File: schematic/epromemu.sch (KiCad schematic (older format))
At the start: 10 parts, among them J1 EPROM Connector, U1 Teensy4.1, U2 74HC245, U3 74HC245, U4 74HC245, U5 74HC245

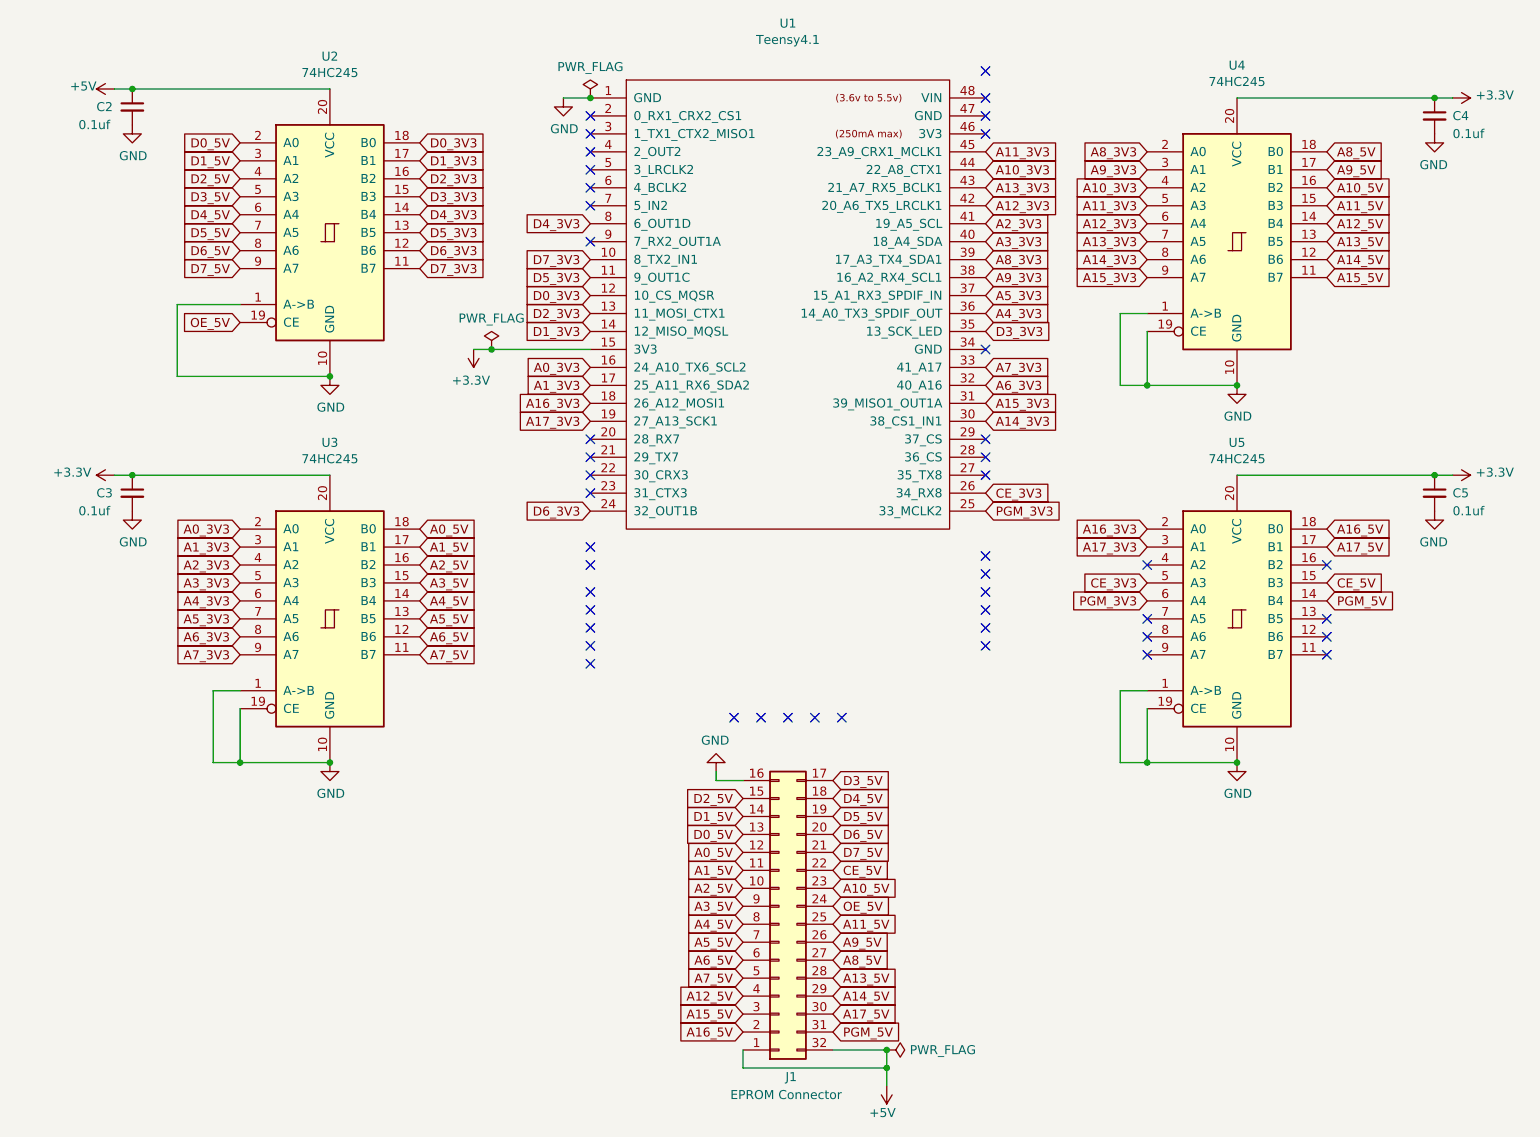
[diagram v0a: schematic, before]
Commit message: updates'
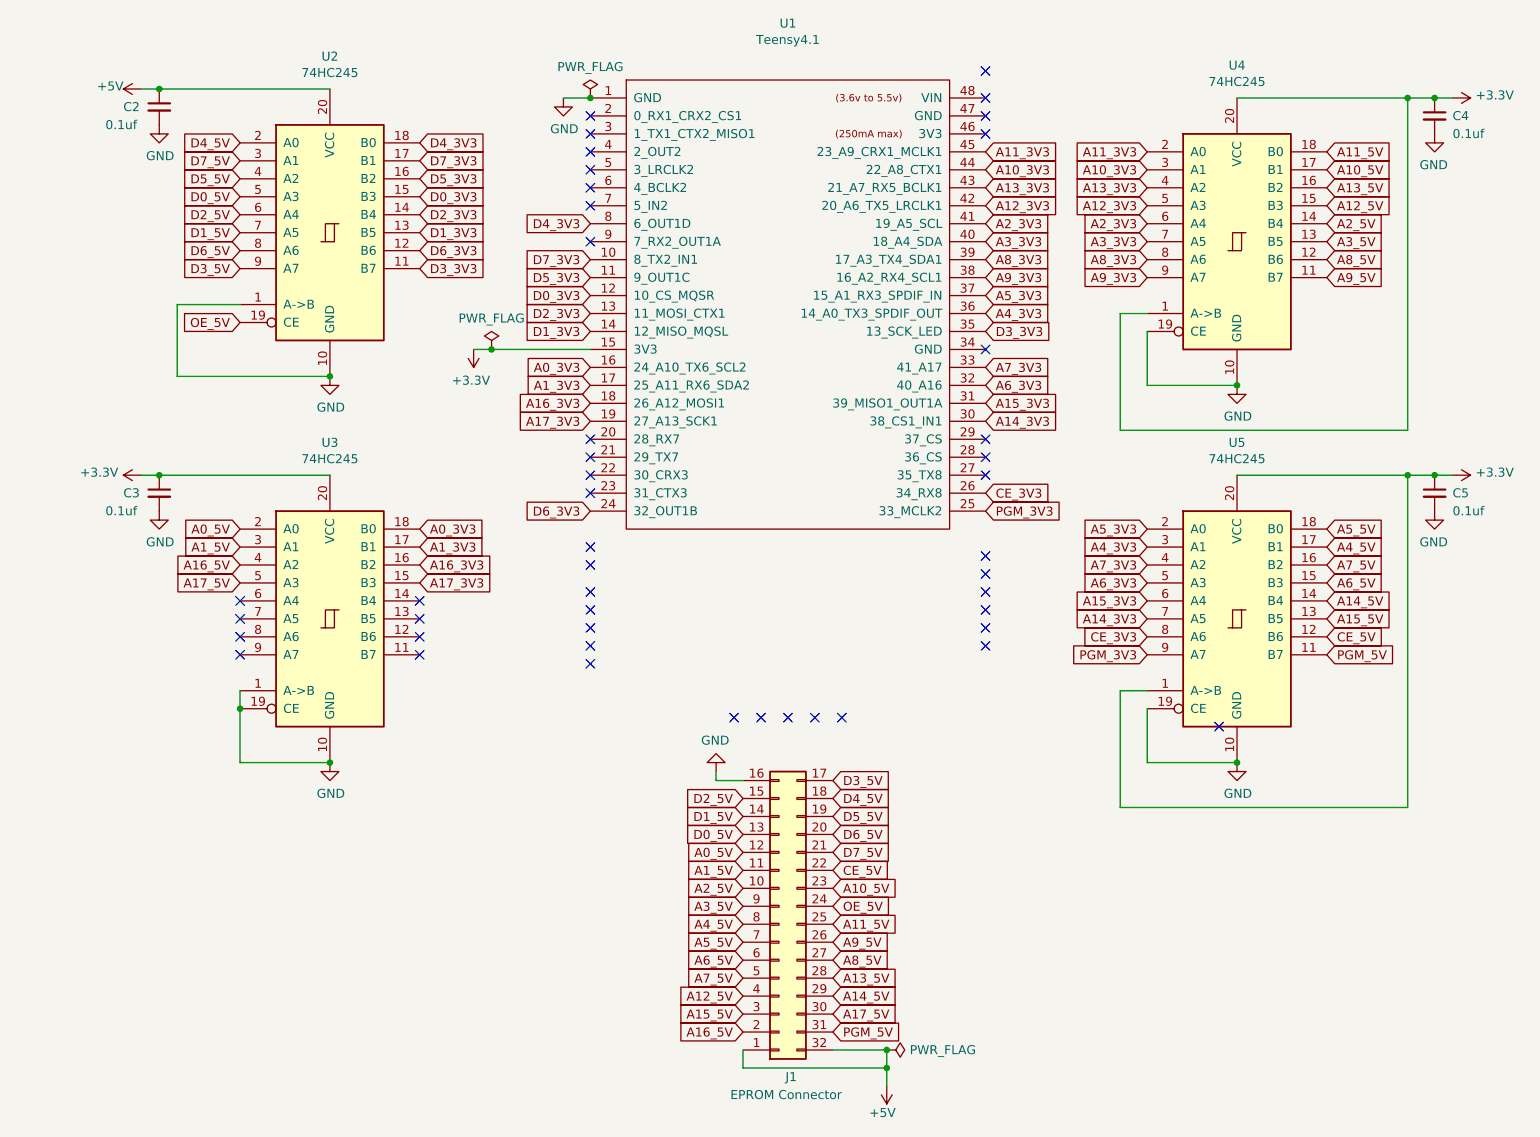
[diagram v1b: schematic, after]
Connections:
- net +3V3: now also U4.1 (A->B), U5.1 (A->B)
- net A0_3V3: now also U3.18 (B0); no longer U3.2 (A0)
- net A0_5V: now also U3.2 (A0); no longer U3.18 (B0)
- net A10_3V3: now also U4.3 (A1); no longer U4.4 (A2)
- net A10_5V: now also U4.17 (B1); no longer U4.16 (B2)
- net A11_3V3: now also U4.2 (A0); no longer U4.5 (A3)
- net A11_5V: now also U4.18 (B0); no longer U4.15 (B3)
- net A12_3V3: now also U4.5 (A3); no longer U4.6 (A4)
- net A12_5V: now also U4.15 (B3); no longer U4.14 (B4)
- net A13_3V3: now also U4.4 (A2); no longer U4.7 (A5)
- net A13_5V: now also U4.16 (B2); no longer U4.13 (B5)
- net A14_3V3: now also U5.7 (A5); no longer U4.8 (A6)
- net A14_5V: now also U5.14 (B4); no longer U4.12 (B6)
- net A15_3V3: now also U5.6 (A4); no longer U4.9 (A7)
- net A15_5V: now also U5.13 (B5); no longer U4.11 (B7)
- net A16_3V3: now also U3.16 (B2); no longer U5.2 (A0)
- net A16_5V: now also U3.4 (A2); no longer U5.18 (B0)
- net A17_3V3: now also U3.15 (B3); no longer U5.3 (A1)
- net A17_5V: now also U3.5 (A3); no longer U5.17 (B1)
- net A1_3V3: now also U3.17 (B1); no longer U3.3 (A1)
- net A1_5V: now also U3.3 (A1); no longer U3.17 (B1)
- net A2_3V3: now also U4.6 (A4); no longer U3.4 (A2)
- net A2_5V: now also U4.14 (B4); no longer U3.16 (B2)
- net A3_3V3: now also U4.7 (A5); no longer U3.5 (A3)
- net A3_5V: now also U4.13 (B5); no longer U3.15 (B3)
- net A4_3V3: now also U5.3 (A1); no longer U3.6 (A4)
- net A4_5V: now also U5.17 (B1); no longer U3.14 (B4)
- net A5_3V3: now also U5.2 (A0); no longer U3.7 (A5)
- net A5_5V: now also U5.18 (B0); no longer U3.13 (B5)
- net A6_3V3: now also U5.5 (A3); no longer U3.8 (A6)
- net A6_5V: now also U5.15 (B3); no longer U3.12 (B6)
- net A7_3V3: now also U5.4 (A2); no longer U3.9 (A7)
- net A7_5V: now also U5.16 (B2); no longer U3.11 (B7)
- net A8_3V3: now also U4.8 (A6); no longer U4.2 (A0)
- net A8_5V: now also U4.12 (B6); no longer U4.18 (B0)
- net A9_3V3: now also U4.9 (A7); no longer U4.3 (A1)
- net A9_5V: now also U4.11 (B7); no longer U4.17 (B1)
- net CE_3V3: now also U5.8 (A6); no longer U5.5 (A3)
- net CE_5V: now also U5.12 (B6); no longer U5.15 (B3)
- net D0_3V3: now also U2.15 (B3); no longer U2.18 (B0)
- net D0_5V: now also U2.5 (A3); no longer U2.2 (A0)
- net D1_3V3: now also U2.13 (B5); no longer U2.17 (B1)
- net D1_5V: now also U2.7 (A5); no longer U2.3 (A1)
- net D2_3V3: now also U2.14 (B4); no longer U2.16 (B2)
- net D2_5V: now also U2.6 (A4); no longer U2.4 (A2)
- net D3_3V3: now also U2.11 (B7); no longer U2.15 (B3)
- net D3_5V: now also U2.9 (A7); no longer U2.5 (A3)
- net D4_3V3: now also U2.18 (B0); no longer U2.14 (B4)
- net D4_5V: now also U2.2 (A0); no longer U2.6 (A4)
- net D5_3V3: now also U2.16 (B2); no longer U2.13 (B5)
- net D5_5V: now also U2.4 (A2); no longer U2.7 (A5)
- net D7_3V3: now also U2.17 (B1); no longer U2.11 (B7)
- net D7_5V: now also U2.3 (A1); no longer U2.9 (A7)
- net GND: no longer U4.1 (A->B), U5.1 (A->B)
- net PGM_3V3: now also U5.9 (A7); no longer U5.6 (A4)
- net PGM_5V: now also U5.11 (B7); no longer U5.14 (B4)
- no-connect marks 45 -> 46
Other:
- moved on the sheet: C2, C3

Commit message: final?
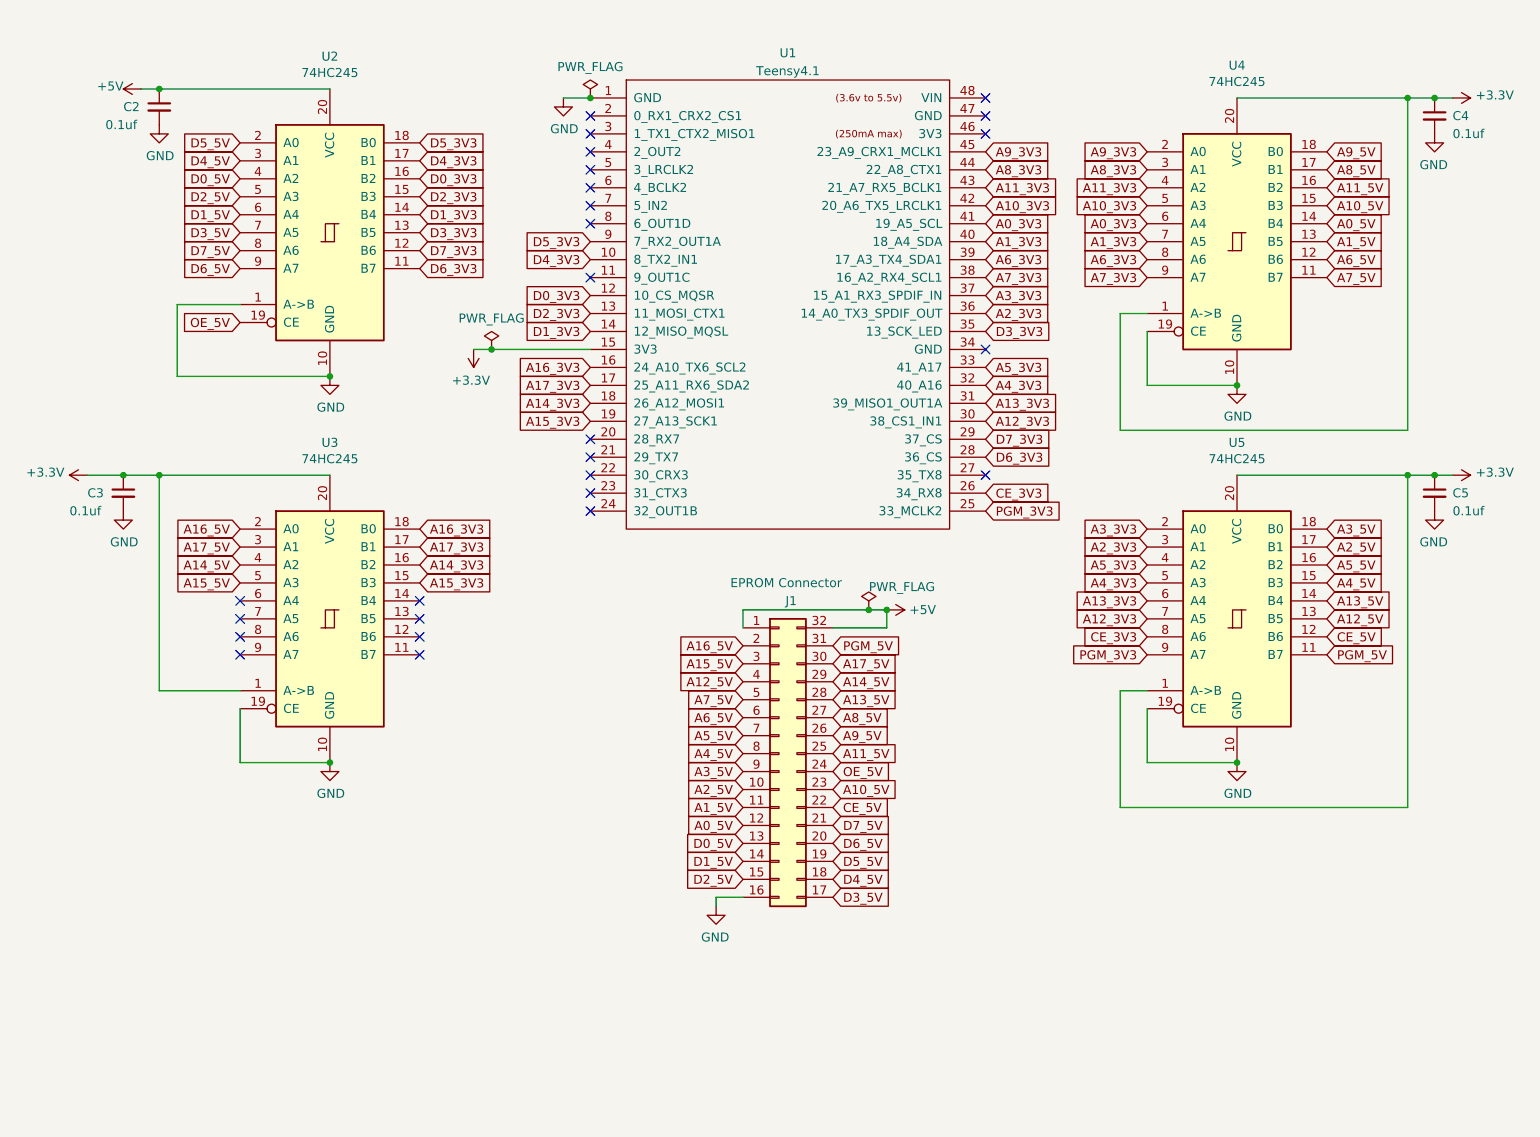
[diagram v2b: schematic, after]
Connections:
- net +3V3: now also U3.1 (A->B)
- net A0_3V3: now also U1.41 (19_A5_SCL), U4.6 (A4); no longer U1.16 (24_A10_TX6_SCL2), U3.18 (B0)
- net A0_5V: now also U4.14 (B4); no longer U3.2 (A0)
- net A10_3V3: now also U1.42 (20_A6_TX5_LRCLK1), U4.5 (A3); no longer U1.44 (22_A8_CTX1), U4.3 (A1)
- net A10_5V: now also U4.15 (B3); no longer U4.17 (B1)
- net A11_3V3: now also U1.43 (21_A7_RX5_BCLK1), U4.4 (A2); no longer U1.45 (23_A9_CRX1_MCLK1), U4.2 (A0)
- net A11_5V: now also U4.16 (B2); no longer U4.18 (B0)
- net A12_3V3: now also U1.30 (38_CS1_IN1), U5.7 (A5); no longer U1.42 (20_A6_TX5_LRCLK1), U4.5 (A3)
- net A12_5V: now also U5.13 (B5); no longer U4.15 (B3)
- net A13_3V3: now also U1.31 (39_MISO1_OUT1A), U5.6 (A4); no longer U1.43 (21_A7_RX5_BCLK1), U4.4 (A2)
- net A13_5V: now also U5.14 (B4); no longer U4.16 (B2)
- net A14_3V3: now also U1.18 (26_A12_MOSI1), U3.16 (B2); no longer U1.30 (38_CS1_IN1), U5.7 (A5)
- net A14_5V: now also U3.4 (A2); no longer U5.14 (B4)
- net A15_3V3: now also U1.19 (27_A13_SCK1), U3.15 (B3); no longer U1.31 (39_MISO1_OUT1A), U5.6 (A4)
- net A15_5V: now also U3.5 (A3); no longer U5.13 (B5)
- net A16_3V3: now also U1.16 (24_A10_TX6_SCL2), U3.18 (B0); no longer U1.18 (26_A12_MOSI1), U3.16 (B2)
- net A16_5V: now also U3.2 (A0); no longer U3.4 (A2)
- net A17_3V3: now also U1.17 (25_A11_RX6_SDA2), U3.17 (B1); no longer U1.19 (27_A13_SCK1), U3.15 (B3)
- net A17_5V: now also U3.3 (A1); no longer U3.5 (A3)
- net A1_3V3: now also U1.40 (18_A4_SDA), U4.7 (A5); no longer U1.17 (25_A11_RX6_SDA2), U3.17 (B1)
- net A1_5V: now also U4.13 (B5); no longer U3.3 (A1)
- net A2_3V3: now also U1.36 (14_A0_TX3_SPDIF_OUT), U5.3 (A1); no longer U1.41 (19_A5_SCL), U4.6 (A4)
- net A2_5V: now also U5.17 (B1); no longer U4.14 (B4)
- net A3_3V3: now also U1.37 (15_A1_RX3_SPDIF_IN), U5.2 (A0); no longer U1.40 (18_A4_SDA), U4.7 (A5)
- net A3_5V: now also U5.18 (B0); no longer U4.13 (B5)
- net A4_3V3: now also U1.32 (40_A16), U5.5 (A3); no longer U1.36 (14_A0_TX3_SPDIF_OUT), U5.3 (A1)
- net A4_5V: now also U5.15 (B3); no longer U5.17 (B1)
- net A5_3V3: now also U1.33 (41_A17), U5.4 (A2); no longer U1.37 (15_A1_RX3_SPDIF_IN), U5.2 (A0)
- net A5_5V: now also U5.16 (B2); no longer U5.18 (B0)
- net A6_3V3: now also U1.39 (17_A3_TX4_SDA1), U4.8 (A6); no longer U1.32 (40_A16), U5.5 (A3)
- net A6_5V: now also U4.12 (B6); no longer U5.15 (B3)
- net A7_3V3: now also U1.38 (16_A2_RX4_SCL1), U4.9 (A7); no longer U1.33 (41_A17), U5.4 (A2)
- net A7_5V: now also U4.11 (B7); no longer U5.16 (B2)
- net A8_3V3: now also U1.44 (22_A8_CTX1), U4.3 (A1); no longer U1.39 (17_A3_TX4_SDA1), U4.8 (A6)
- net A8_5V: now also U4.17 (B1); no longer U4.12 (B6)
- net A9_3V3: now also U1.45 (23_A9_CRX1_MCLK1), U4.2 (A0); no longer U1.38 (16_A2_RX4_SCL1), U4.9 (A7)
- net A9_5V: now also U4.18 (B0); no longer U4.11 (B7)
- net D0_3V3: now also U2.16 (B2); no longer U2.15 (B3)
- net D0_5V: now also U2.4 (A2); no longer U2.5 (A3)
- net D1_3V3: now also U2.14 (B4); no longer U2.13 (B5)
- net D1_5V: now also U2.6 (A4); no longer U2.7 (A5)
- net D2_3V3: now also U2.15 (B3); no longer U2.14 (B4)
- net D2_5V: now also U2.5 (A3); no longer U2.6 (A4)
- net D3_3V3: now also U2.13 (B5); no longer U2.11 (B7)
- net D3_5V: now also U2.7 (A5); no longer U2.9 (A7)
- net D4_3V3: now also U1.10 (8_TX2_IN1), U2.17 (B1); no longer U1.8 (6_OUT1D), U2.18 (B0)
- net D4_5V: now also U2.3 (A1); no longer U2.2 (A0)
- net D5_3V3: now also U1.9 (7_RX2_OUT1A), U2.18 (B0); no longer U1.11 (9_OUT1C), U2.16 (B2)
- net D5_5V: now also U2.2 (A0); no longer U2.4 (A2)
- net D6_3V3: now also U1.28 (36_CS), U2.11 (B7); no longer U1.24 (32_OUT1B), U2.12 (B6)
- net D6_5V: now also U2.9 (A7); no longer U2.8 (A6)
- net D7_3V3: now also U1.29 (37_CS), U2.12 (B6); no longer U1.10 (8_TX2_IN1), U2.17 (B1)
- net D7_5V: now also U2.8 (A6); no longer U2.3 (A1)
- net GND: no longer U3.1 (A->B)
- no-connect marks 46 -> 26
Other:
- moved on the sheet: C3, J1
